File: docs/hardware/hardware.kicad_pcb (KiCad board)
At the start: 2 copper layers, 1.4 x 13 mm, 8 parts, among them J1 BASYS_JA, J2 AudioJack2, J6 BASYS_JB, J7 GAMEPAD_1, J8 GAMEPAD_2

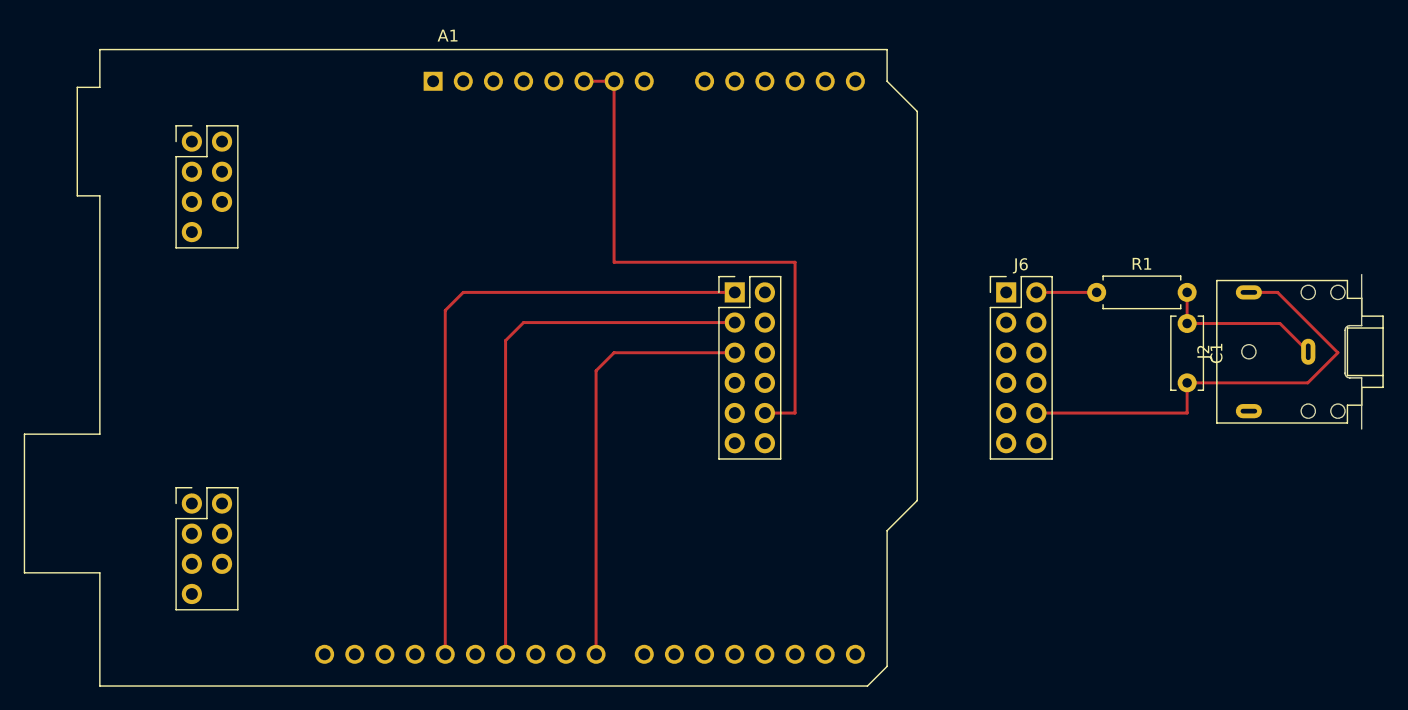
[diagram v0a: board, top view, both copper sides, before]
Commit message: WIP ppu testing
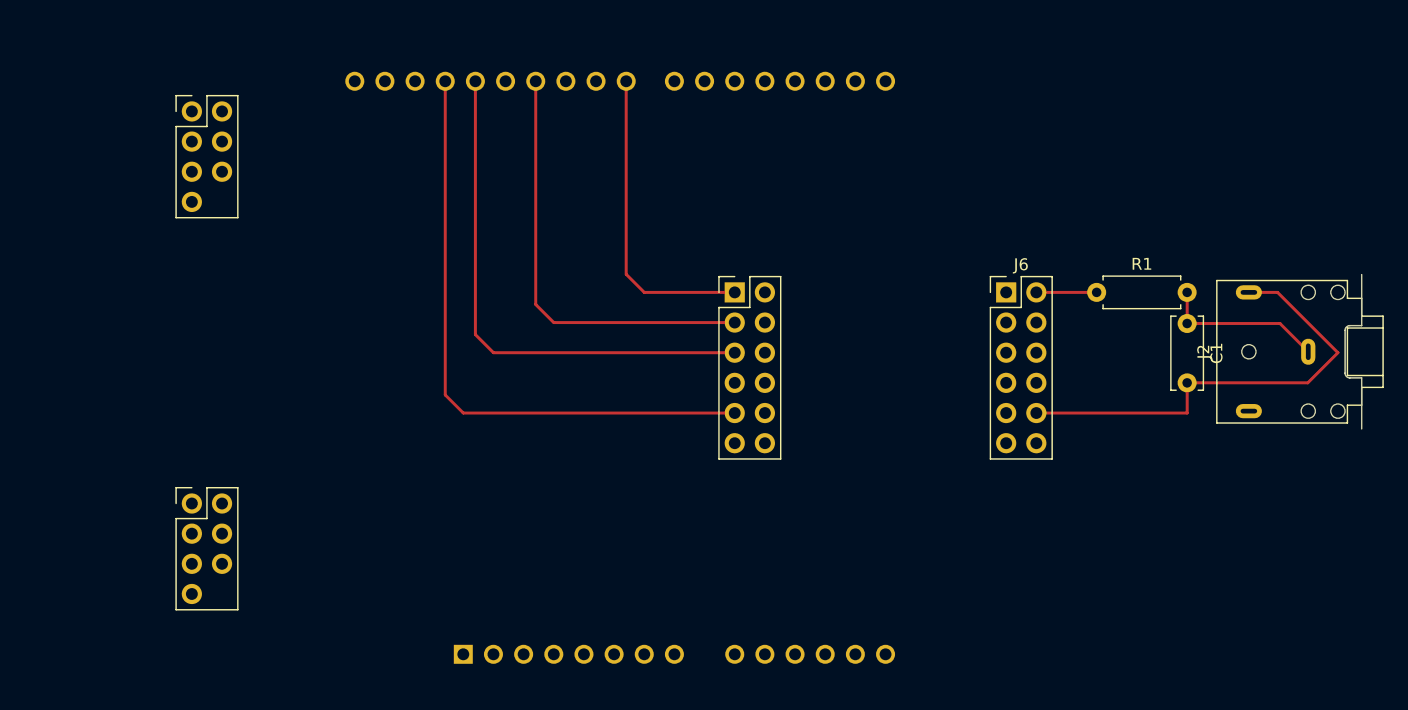
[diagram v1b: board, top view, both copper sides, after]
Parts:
- A1: moved to B.Cu
- moved A1 48.3 mm to (53.3, 66.0)
- moved J7 33.0 mm to (30.5, 20.3)
- moved J8 30.5 mm to (30.5, 53.3)
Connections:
- J1 pad 1: SPI_CLK -> PPU_VRAM_WEN
- J1 pad 3: PPU_VRAM_WEN -> SPI_CLK
- J1 pad 5: (no net) -> GND
- J6 pad 5: unconnected-(J6-Pin_5-Pad5) -> GND
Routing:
- net PPU_VRAM_WEN: track 36.2 -> 26.0 mm
- net SPI_MOSI: track 46.3 -> 36.2 mm
- net SPI_CLK: track 54.0 -> 43.8 mm
- net GND: track 86.9 -> 90.0 mm
